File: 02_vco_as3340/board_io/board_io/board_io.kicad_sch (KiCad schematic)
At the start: 9 parts, among them J1 Header 1, J2 Header 2, SW2 SW_SPDT

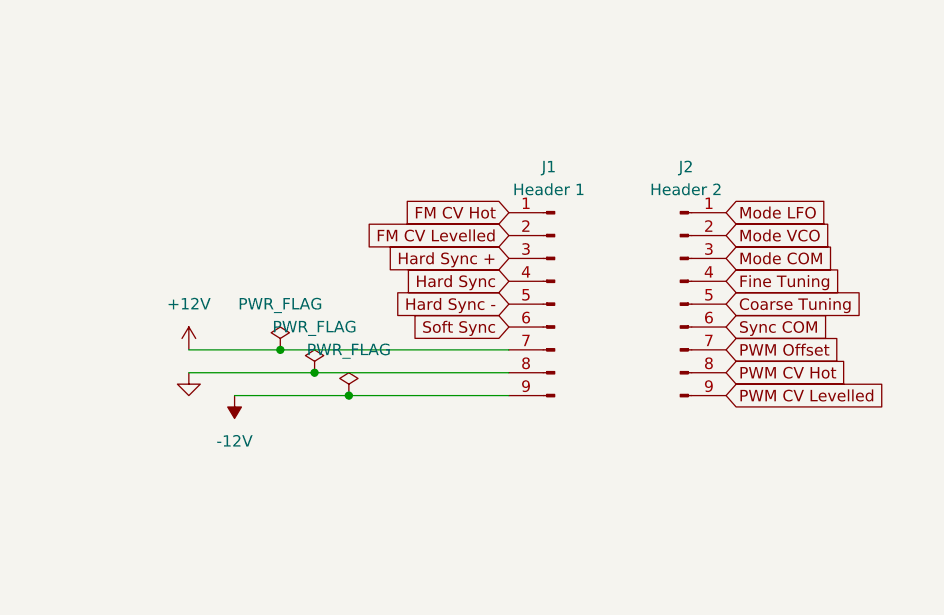
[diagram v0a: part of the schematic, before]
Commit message: routed everyting
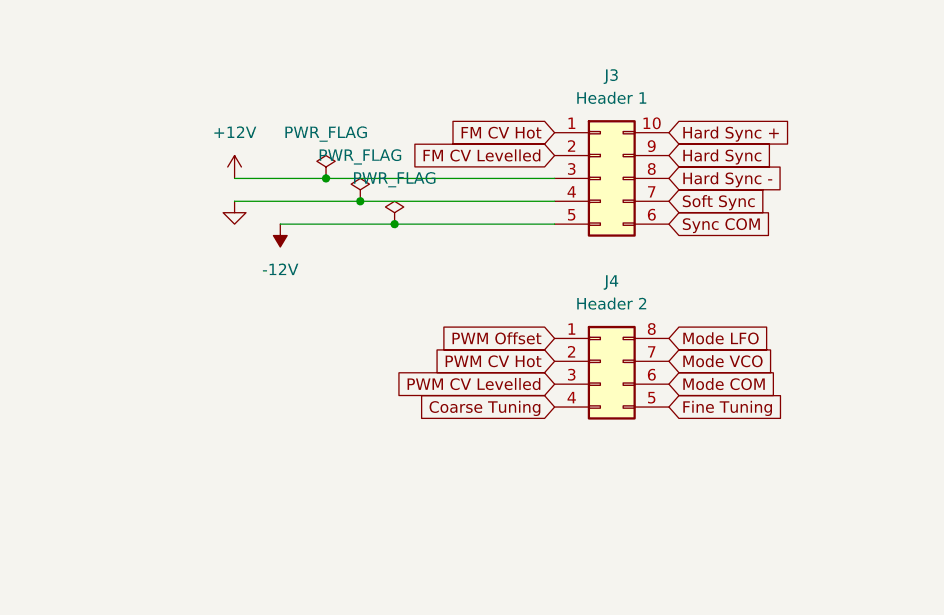
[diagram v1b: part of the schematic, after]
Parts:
- removed J1: Header 1, Connector_PinHeader_2.54mm:PinHeader_1x09_P2.54mm_Vertical, symbol Connector:Conn_01x09_Pin
- removed J2: Header 2, Connector_PinHeader_2.54mm:PinHeader_1x09_P2.54mm_Vertical, symbol Connector:Conn_01x09_Pin
- added J3: Header 1, Connector_PinHeader_2.54mm:PinHeader_2x05_P2.54mm_Vertical, symbol Connector_Generic:Conn_02x05_Counter_Clockwise
- added J4: Header 2, Connector_PinHeader_2.54mm:PinHeader_2x04_P2.54mm_Vertical, symbol Connector_Generic:Conn_02x04_Counter_Clockwise
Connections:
- net +12V: now also J3.3 (Pin_3)
- net -12V: now also J3.5 (Pin_5)
- net Coarse Tuning: now also J4.4 (Pin_4)
- net FM CV Hot: now also J3.1 (Pin_1)
- net FM CV Levelled: now also J3.2 (Pin_2)
- net Fine Tuning: now also J4.5 (Pin_5)
- net GND: now also J3.4 (Pin_4)
- net Hard Sync: now also J3.9 (Pin_9)
- net Hard Sync +: now also J3.10 (Pin_10)
- net Hard Sync -: now also J3.8 (Pin_8)
- net Mode COM: now also J4.6 (Pin_6)
- net Mode LFO: now also J4.8 (Pin_8)
- net Mode VCO: now also J4.7 (Pin_7)
- net PWM CV Hot: now also J4.2 (Pin_2)
- net PWM CV Levelled: now also J4.3 (Pin_3)
- net PWM Offset: now also J4.1 (Pin_1)
- net Soft Sync: now also J3.7 (Pin_7)
- net Sync COM: now also J3.6 (Pin_6)
